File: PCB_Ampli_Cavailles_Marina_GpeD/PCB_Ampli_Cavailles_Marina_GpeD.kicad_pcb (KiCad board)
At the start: 2 copper layers, 52 parts, among them J2 Conn_01x02, J3 Conn_01x03, Q1 2N2907, Q10 TIP32, Q11 BD138, Q12 TIP31, Q13 2N2222, Q2 2N2907, Q3 2N2907, Q4 2N2222, Q5 2N2222, Q6 2N2907, Q7 2N2907, Q8 BD139, Q9 BD139, U1 Relay_1CT, U2 Jack_Mono

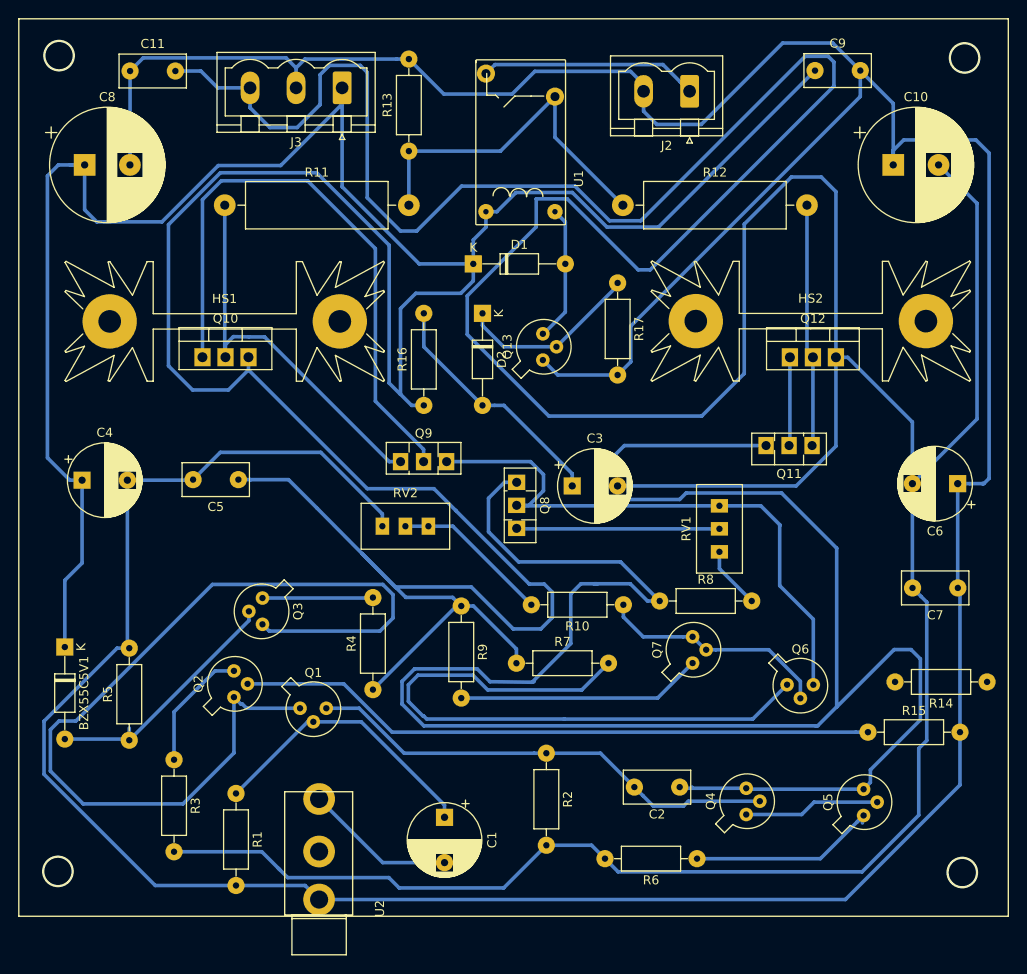
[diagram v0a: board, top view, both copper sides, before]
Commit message: Routage fini
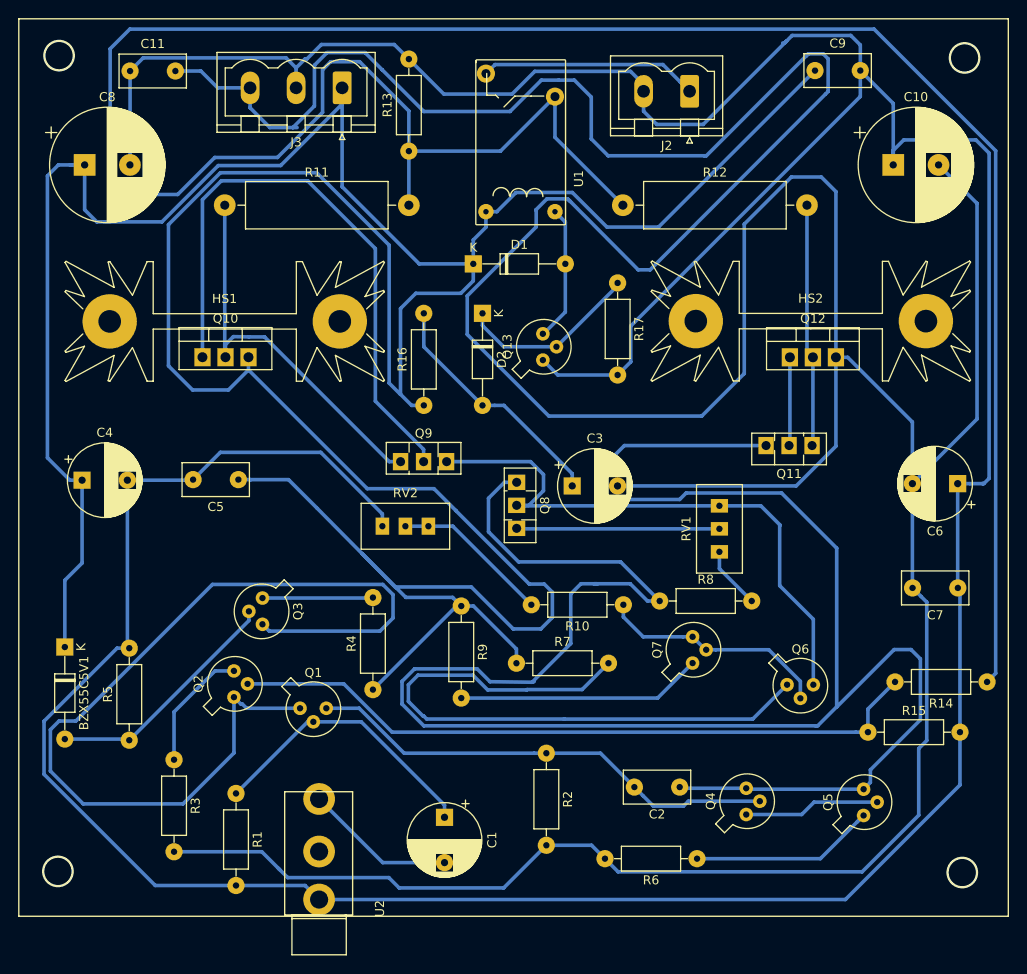
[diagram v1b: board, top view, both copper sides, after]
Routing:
- net Net-(R11-Pad2): track 39.7 -> 266.8 mm
- net -12V: track 478.9 -> 468.5 mm
- net Net-(Q2-Pad2): track 70.7 -> 77.5 mm
- net GND: track 441.2 -> 445.4 mm
- net Net-(BZX55C5V1-Pad2): track 28.2 -> 26.7 mm
- net Net-(Q5-Pad1): track 22.5 -> 21.4 mm

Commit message: Changes
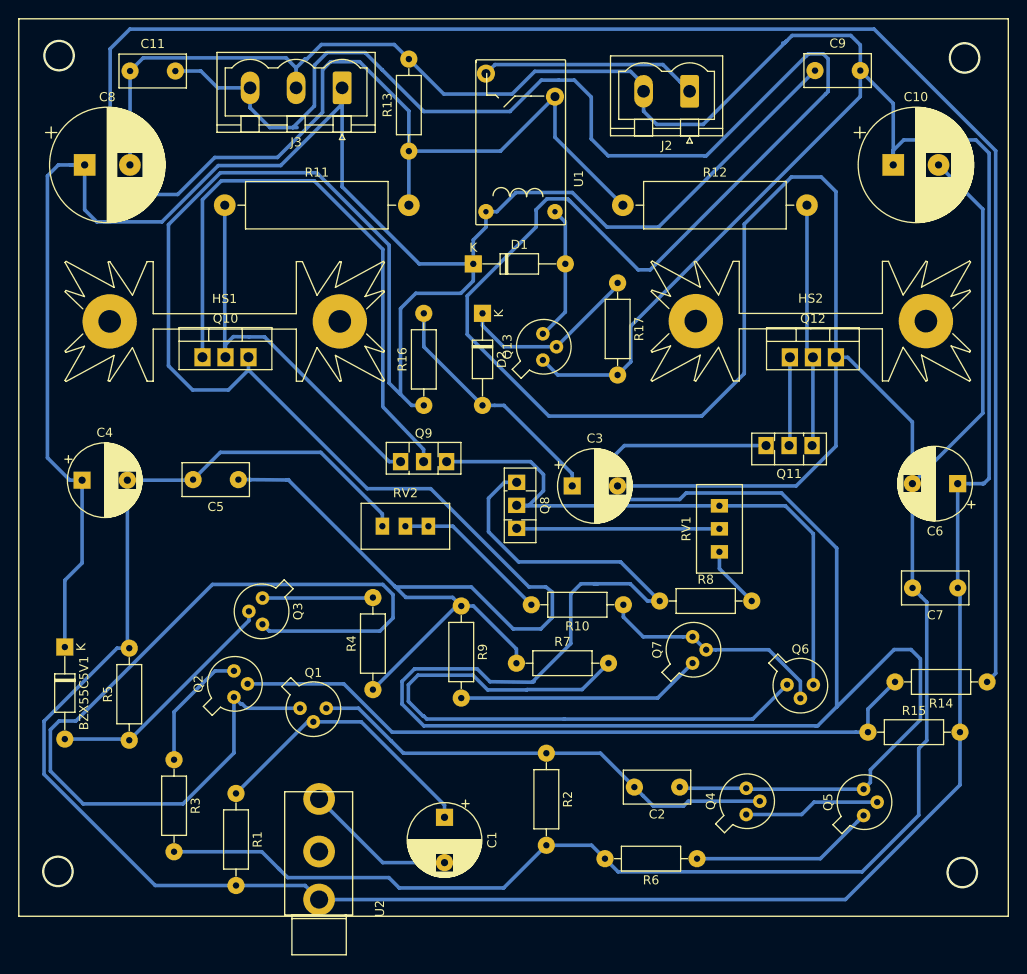
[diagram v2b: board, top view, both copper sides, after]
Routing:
- net +12V: track 407.4 -> 402.4 mm
- net Net-(Q6-Pad3): track 65.9 -> 67.4 mm
- net -12V: track 468.5 -> 469.0 mm
